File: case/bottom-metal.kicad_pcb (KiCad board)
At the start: 2 copper layers, 135 x 95.7 mm, 6 parts

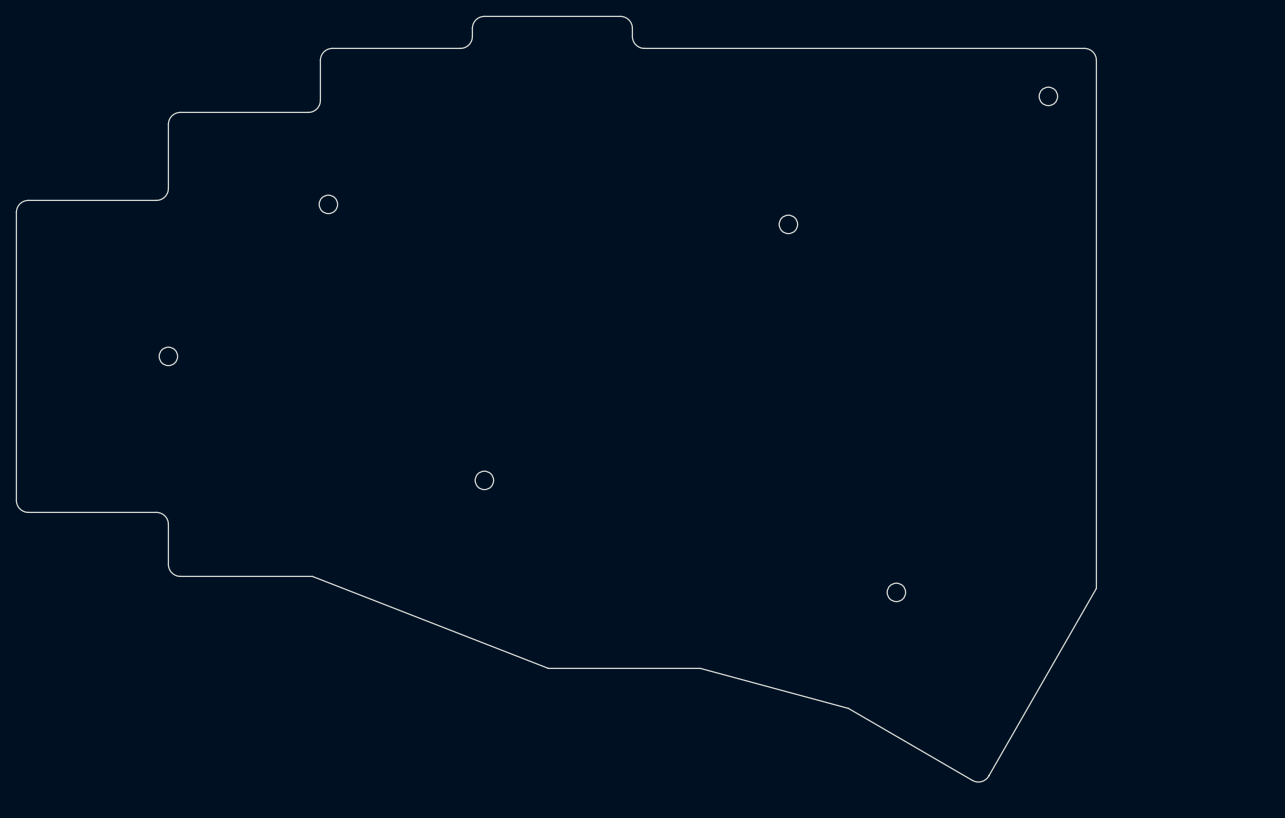
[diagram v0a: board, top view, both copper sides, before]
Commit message: update case files
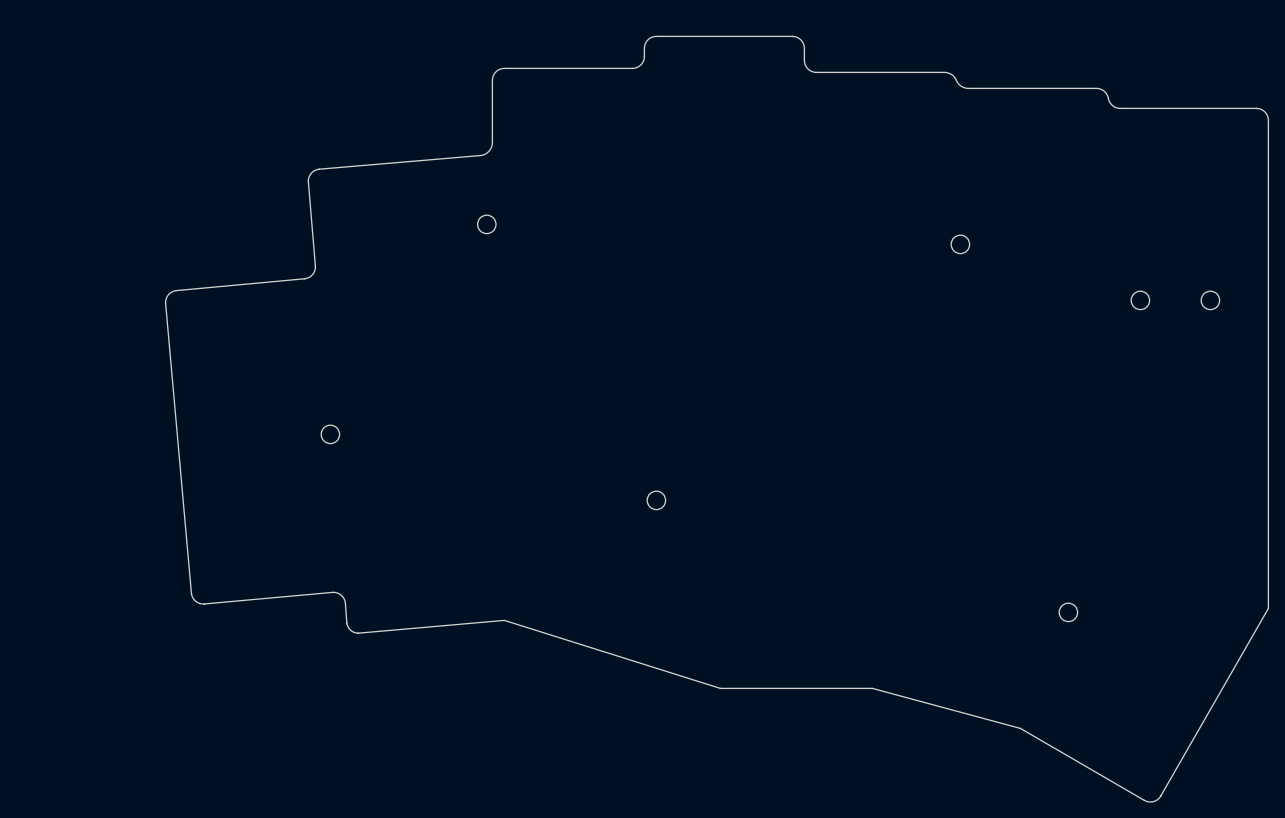
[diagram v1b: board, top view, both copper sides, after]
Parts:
- removed the H5 at (195.0, 61.0)
- removed the H5 at (162.5, 77.0)
- added H5: MountingHole, kbd:thread_m2, F.Cu at (184.0, 79.5)
- added H6: MountingHole, kbd:thread_m2, F.Cu at (206.5, 86.5)
- added H7: MountingHole, kbd:thread_m2, F.Cu at (215.2, 86.5)
- moved H3 22.5 mm to (105.2, 103.2), turned to 5 degrees
- moved H2 21.6 mm to (197.5, 125.5)
- moved H4 21.6 mm to (146.0, 111.5)
- moved H1 20.0 mm to (124.8, 77.0)
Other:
- board size 135 x 95.7 mm -> 137.8 x 95.7 mm
